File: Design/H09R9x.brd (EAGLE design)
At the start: 34.6 x 30 mm, 24 parts, among them P1 HEXABIT_17.32, U1 STM32F091CBU6, U2 TSD305-1C55, X1 XTALL_CSTCE8M00G52

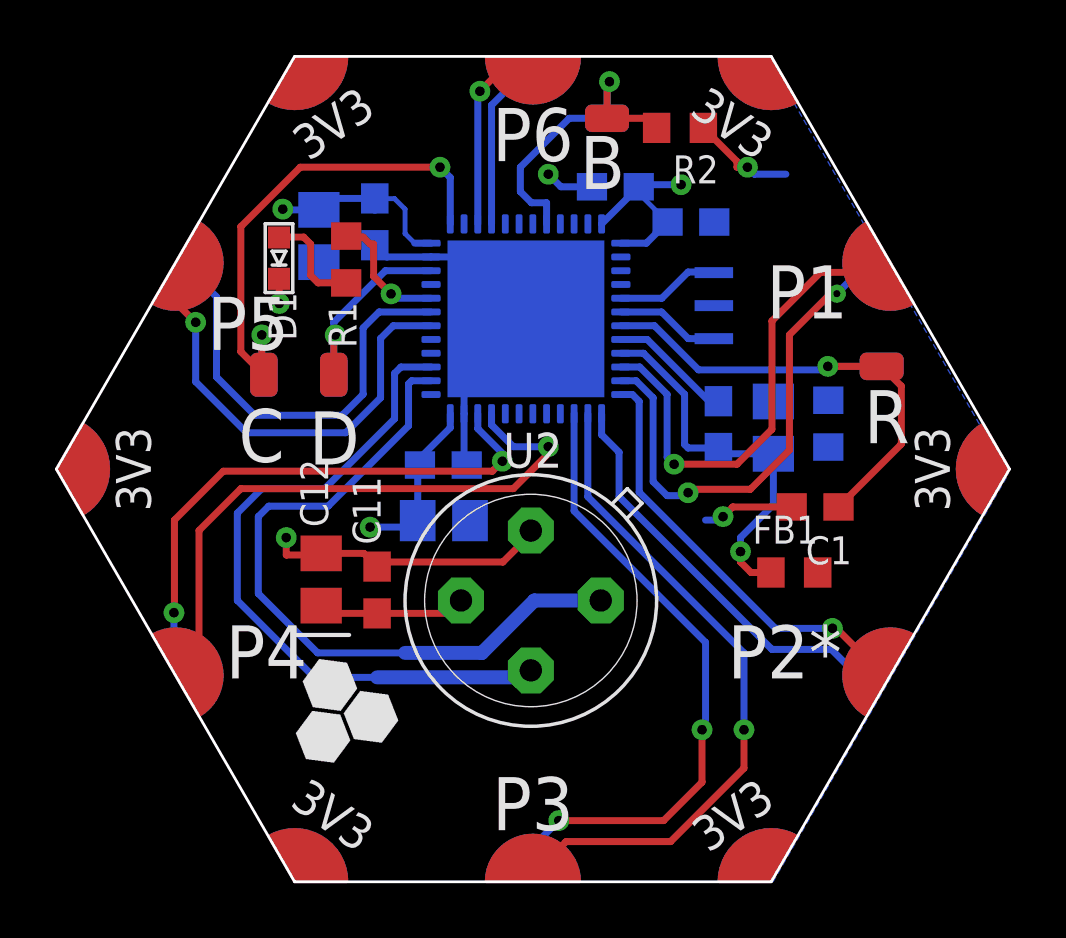
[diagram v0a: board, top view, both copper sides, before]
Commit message: edit brd
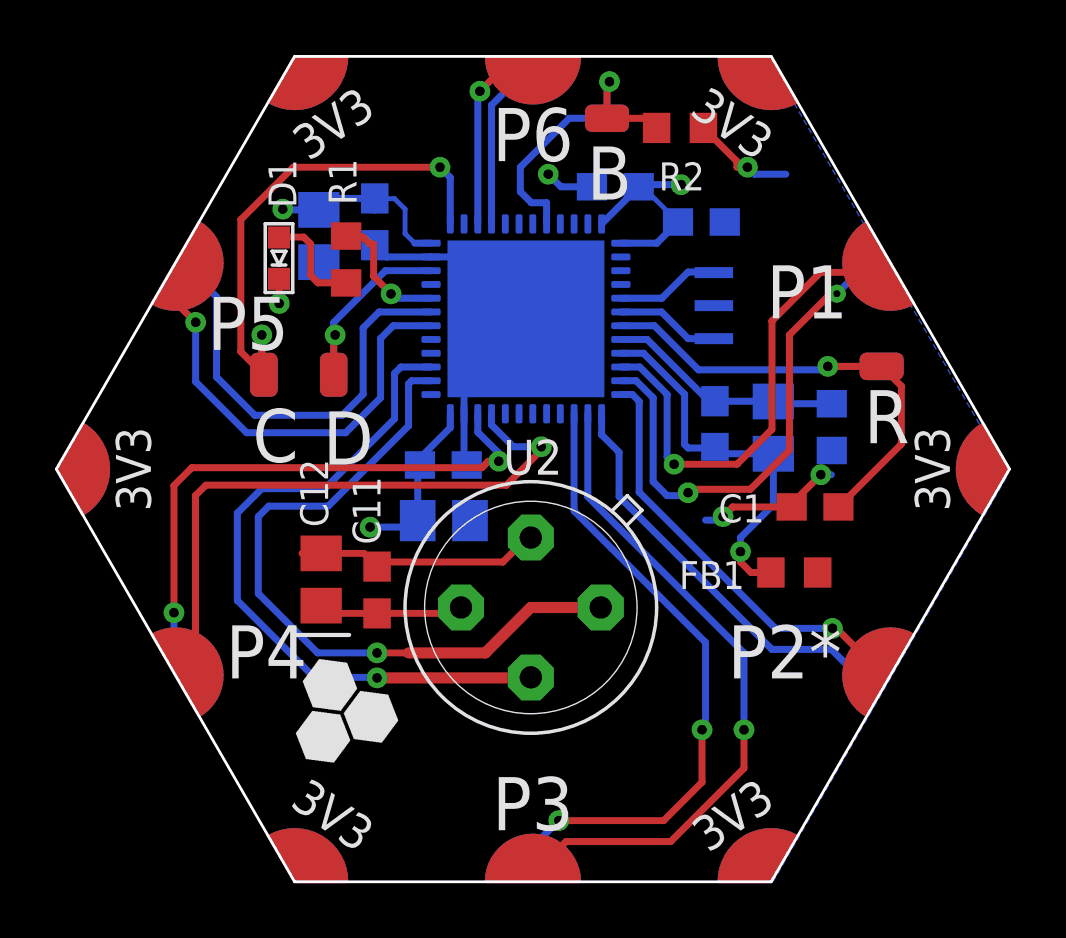
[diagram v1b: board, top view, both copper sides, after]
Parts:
- moved C9 0.38 mm to (40.7, 43.6)
- moved U2 0.25 mm to (34.5, 29.6)
- moved R3 0.18 mm to (45.5, 36.1)
- moved C5 0.13 mm to (41.2, 36.2)
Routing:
- net VSSA: track 4.47 -> 8.63 mm
- net USART2_RX: track 16.7 -> 15.5 mm
- net USART6_TX: track 25.2 -> 24.3 mm
- net I2C2_SDA: track 26.0 -> 25.2 mm, vias 0 -> 1
- net GND: track 35.6 -> 36.3 mm
- net VDD: track 26.0 -> 26.5 mm
- net I2C2_SCL: track 26.1 -> 26.0 mm, vias 0 -> 1
